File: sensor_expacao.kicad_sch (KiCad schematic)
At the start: 53 parts, among them J10 Conn_01x11_Socket, J11 Micro_SD_Card, J12 Conn_01x10, J13 ntc, J8 Micro_SD_Card, J9 Conn_01x15_Pin, Q6 NMOS, Q7 NMOS, Q8 NMOS, U10 74HC4051, U9 SRV05-4

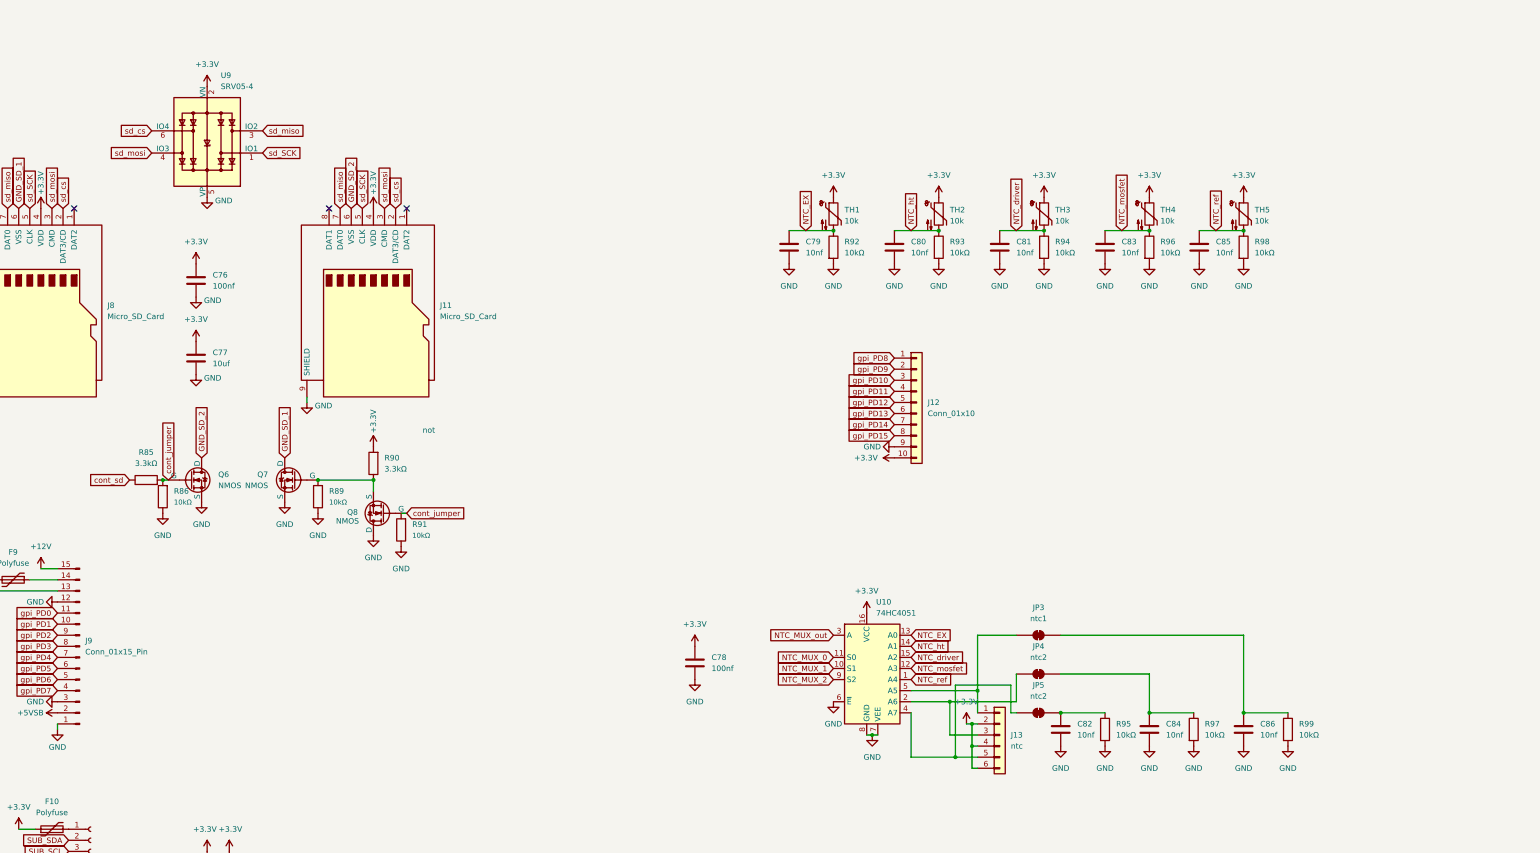
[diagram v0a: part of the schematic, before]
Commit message: 29082026/I
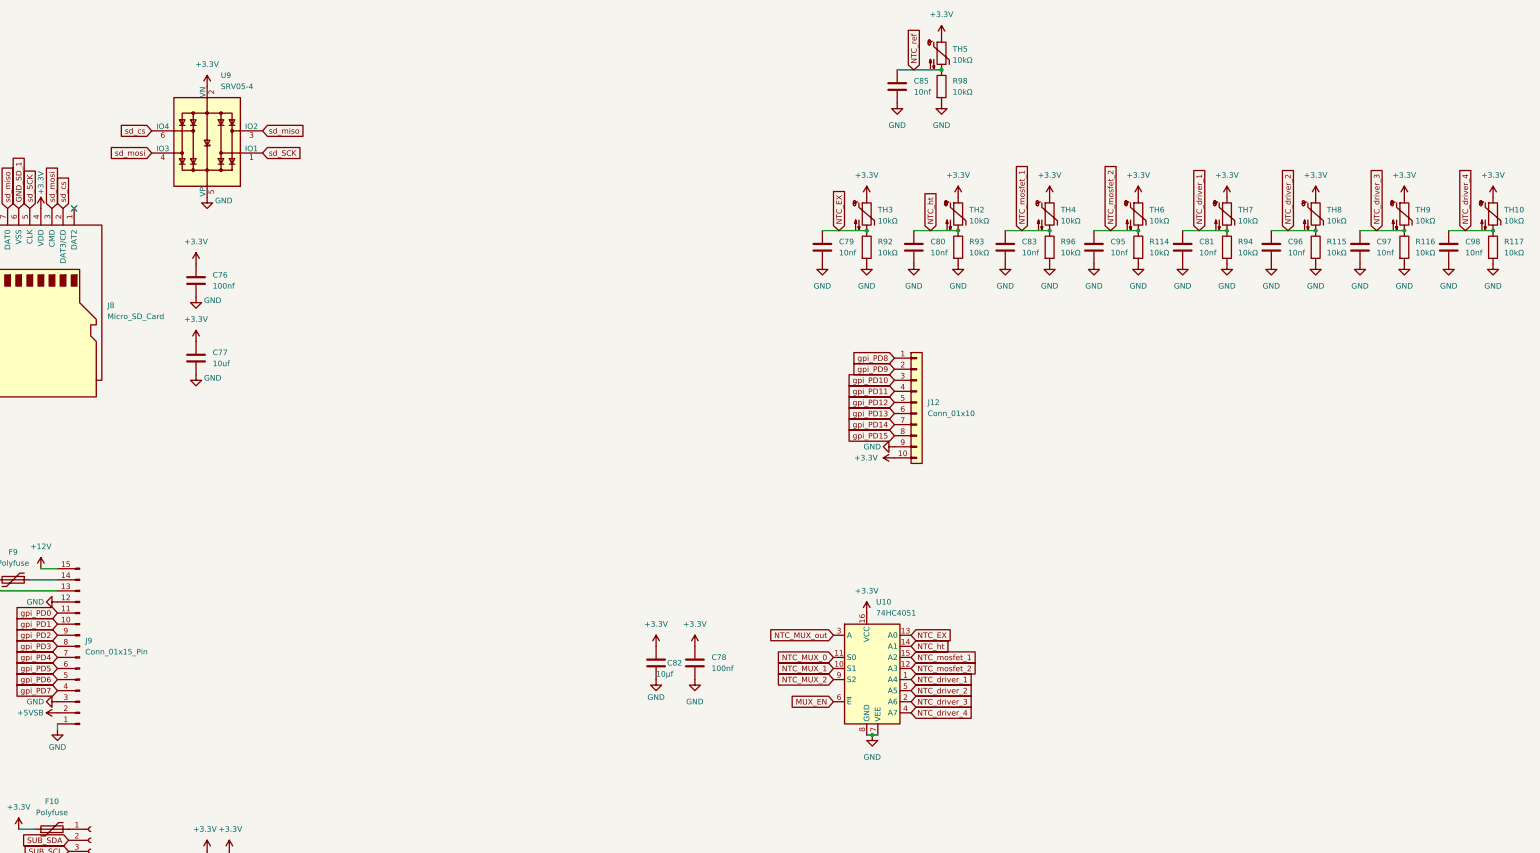
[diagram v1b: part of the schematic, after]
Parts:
- removed C84, C86: 10nf, symbol Device:C
- removed J11: Micro_SD_Card, symbol Connector:Micro_SD_Card
- removed J13: ntc, symbol Connector_Generic:Conn_01x06
- removed JP3: ntc1, symbol Jumper:SolderJumper_2_Bridged
- removed JP4, JP5: ntc2, symbol Jumper:SolderJumper_2_Bridged
- removed Q6, Q7, Q8: NMOS, symbol Simulation_SPICE:NMOS
- removed R85, R90: 3.3kΩ, symbol Device:R
- removed R86, R89, R91, R95, R97, R99: 10kΩ, symbol Device:R
- removed TH1: 10k, symbol Device:Thermistor_NTC
- added C95, C96, C97, C98: 10nf, symbol Device:C
- added R114, R115, R116, R117: 10kΩ, symbol Device:R
- added TH10, TH6, TH7, TH8, TH9: 10kΩ, Resistor_SMD:R_0603_1608Metric, symbol Device:Thermistor_NTC
- C70, C71, C72, C76, C78: jlc_pcb: C346191 -> C307348; mouser: (none) -> 187-CL10B104KB8WPNC; mpn CL10B104KB8NFNC -> CL10B104KB8WPNC
- C82: value 10nf -> 10µf
- J8: footprint (none) -> Connector_Card:microSD_HC_Molex_47219-2001; jlc_pcb: (none) -> C164170; mouser: (none) -> 538-47219-2001; mpn (none) -> 472192001
- TH2, TH3, TH4: value 10k -> 10kΩ; footprint (none) -> Resistor_SMD:R_0603_1608Metric; jlc_pcb: (none) -> C13564; mouser: (none) -> 81-NCP18XH103F03RB; mpn (none) -> NCP18XH103F03RB
- TH5: value 10k -> 10kΩ
- U10: footprint Package_DIP:DIP-16_W7.62mm -> Package_SO:SOIC-16_3.9x9.9mm_P1.27mm; mouser: (none) -> 771-74HC4051D-T
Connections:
- net +3.3V: now also C82.1, TH10.1, TH6.1, TH7.1, TH8.1, TH9.1
- net GND: now also C95.2, C96.2, C97.2, C98.2, R114.2, R115.2, R116.2, R117.2; no longer U10.6 (~{E})
- net NTC_EX: now also TH3.2
- net NTC_ref: no longer U10.1 (A4)
- net NTC_driver_2: now reaches U10.5 (A5)
- net NTC_driver_2: now also C96.1, R115.1, TH8.2
- net NTC_driver_3: now reaches U10.2 (A6)
- net NTC_driver_3: now also C97.1, R116.1, TH9.2
- net NTC_driver_4: now reaches U10.4 (A7)
- net NTC_driver_4: now also C98.1, R117.1, TH10.2
- net NTC_driver renamed NTC_driver_1
- net NTC_driver_1: now also U10.1 (A4), TH7.2; no longer TH3.2, U10.15 (A2)
- net NTC_mosfet renamed NTC_mosfet_1
- net NTC_mosfet_1: now also U10.15 (A2); no longer U10.12 (A3)
- new net MUX_EN: U10.6 (~{E})
- new net NTC_mosfet_2: C95.1, R114.1, TH6.2, U10.12 (A3)
- no-connect marks 4 -> 2
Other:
- note removed: "not"
- moved on the sheet: C79, C80, C81, C83, C85, R92, R93, R94, R96, R98, TH2
